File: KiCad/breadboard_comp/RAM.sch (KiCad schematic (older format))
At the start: 19 parts, among them SW9 SW_Push, U100 74LS00, U101 74LS245, U102 74LS245, U103 IDT6116SA, U104 IDT6116SA, U105 74LS00, U106 74LS245, U107 74LS245, U28 74LS08, U37 74LS32, U38 74LS08, U66 74LS00, U97 74LS08, U98 74LS32, U99 74LS08

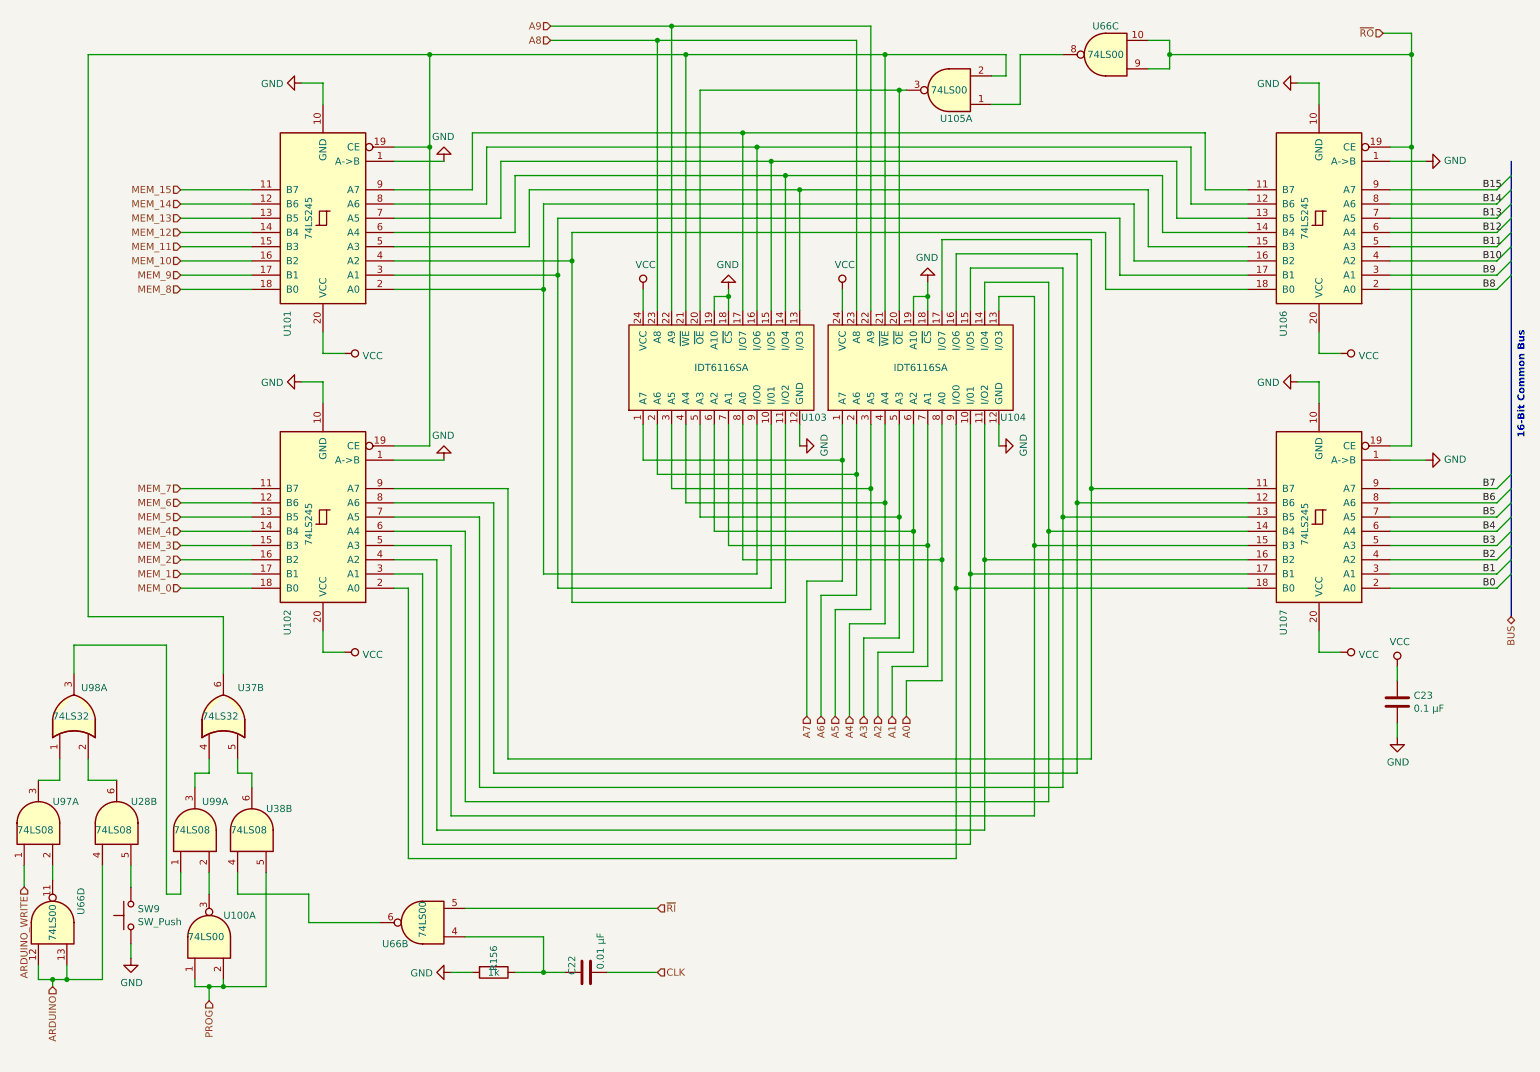
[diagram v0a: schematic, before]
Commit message: Computer built
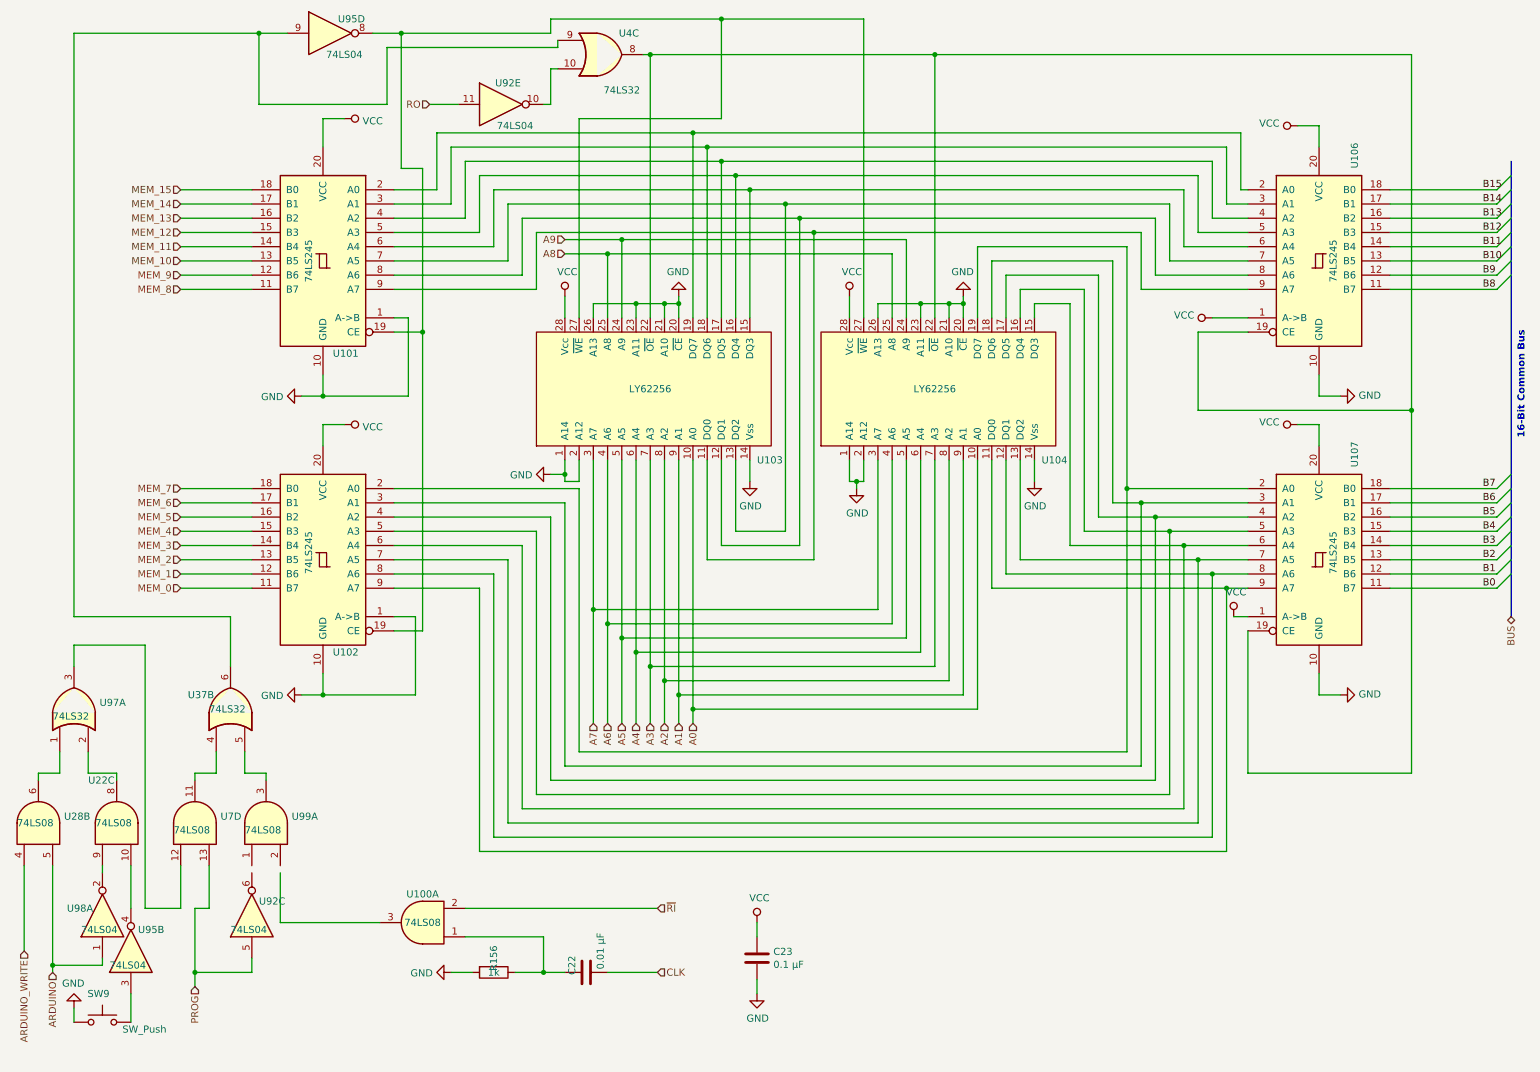
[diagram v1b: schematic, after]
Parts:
- removed U100, U105, U66: 74LS00, symbol 74xx:74LS00
- removed U103, U104: IDT6116SA, Package_DIP:DIP-24_W10.16mm_LongPads, symbol IDT_RAM:IDT6116SA
- removed U38, U97: 74LS08, symbol 74xx:74LS08
- removed U98: 74LS32, symbol 74xx:74LS32
- added U100, U22, U7: 74LS08, symbol 74xx:74LS08
- added U103, U104: LY62256, Package_DIP:DIP-28_W15.24mm, symbol IDT_RAM:LY62256
- added U4, U97: 74LS32, symbol 74xx:74LS32
- added U92, U95, U98: 74LS04, symbol 74xx:74LS04
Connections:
- net A0: now also U103.10 (A0), U104.10 (A0)
- net A1: now also U103.9 (A1), U104.9 (A1)
- net A2: now also U103.8 (A2), U104.8 (A2)
- net A3: now also U103.7 (A3), U104.7 (A3)
- net A4: now also U103.6 (A4), U104.6 (A4)
- net A5: now also U103.5 (A5), U104.5 (A5)
- net A6: now also U103.4 (A6), U104.4 (A6)
- net A7: now also U103.3 (A7), U104.3 (A7)
- net A8: now also U103.25 (A8), U104.25 (A8)
- net A9: now also U103.24 (A9), U104.24 (A9)
- net ARDUINO: now also U28.5, U98.1; no longer U28.4
- net ARDUINO_WRITE: now also U28.4
- net B0: now also U107.11 (B7); no longer U107.2 (A0)
- net B1: now also U107.12 (B6); no longer U107.3 (A1)
- net B10: now also U106.13 (B5); no longer U106.4 (A2)
- net B11: now also U106.14 (B4); no longer U106.5 (A3)
- net B12: now also U106.15 (B3); no longer U106.6 (A4)
- net B13: now also U106.16 (B2); no longer U106.7 (A5)
- net B14: now also U106.17 (B1); no longer U106.8 (A6)
- net B15: now also U106.18 (B0); no longer U106.9 (A7)
- net B2: now also U107.13 (B5); no longer U107.4 (A2)
- net B3: now also U107.14 (B4); no longer U107.5 (A3)
- net B4: now also U107.15 (B3); no longer U107.6 (A4)
- net B5: now also U107.16 (B2); no longer U107.7 (A5)
- net B6: now also U107.17 (B1); no longer U107.8 (A6)
- net B7: now also U107.18 (B0); no longer U107.9 (A7)
- net B8: now also U106.11 (B7); no longer U106.2 (A0)
- net B9: now also U106.12 (B6); no longer U106.3 (A1)
- net GND: now also U103.1 (A14), U103.14 (Vss), U103.2 (A12), U103.20 (~CE), U103.21 (A10), U103.23 (A11), U103.26 (A13), U104.1 (A14), U104.14 (Vss), U104.2 (A12), U104.20 (~CE), U104.21 (A10), U104.23 (A11), U104.26 (A13); no longer U106.1 (A->B), U107.1 (A->B)
- net MEM_0: now also U102.11 (B7); no longer U102.18 (B0)
- net MEM_1: now also U102.12 (B6); no longer U102.17 (B1)
- net MEM_10: now also U101.13 (B5); no longer U101.16 (B2)
- net MEM_11: now also U101.14 (B4); no longer U101.15 (B3)
- net MEM_12: now also U101.15 (B3); no longer U101.14 (B4)
- net MEM_13: now also U101.16 (B2); no longer U101.13 (B5)
- net MEM_14: now also U101.17 (B1); no longer U101.12 (B6)
- net MEM_15: now also U101.18 (B0); no longer U101.11 (B7)
- net MEM_2: now also U102.13 (B5); no longer U102.16 (B2)
- net MEM_3: now also U102.14 (B4); no longer U102.15 (B3)
- net MEM_4: now also U102.15 (B3); no longer U102.14 (B4)
- net MEM_5: now also U102.16 (B2); no longer U102.13 (B5)
- net MEM_6: now also U102.17 (B1); no longer U102.12 (B6)
- net MEM_7: now also U102.18 (B0); no longer U102.11 (B7)
- net MEM_8: now also U101.11 (B7); no longer U101.18 (B0)
- net MEM_9: now also U101.12 (B6); no longer U101.17 (B1)
- net PROG: now also U7.13, U92.5
- net VCC: now also U106.1 (A->B), U107.1 (A->B), U103.28 (Vcc), U104.28 (Vcc)
- net ~RI: now also U100.2
- net at U101.3 (A1): now also U106.3 (A1), U103.18 (DQ6); no longer U106.17 (B1)
- net at U101.4 (A2): now also U106.4 (A2), U103.17 (DQ5); no longer U106.18 (B0)
- net at U101.5 (A3): now also U106.5 (A3), U103.16 (DQ4); no longer U106.15 (B3)
- net at U101.6 (A4): now also U106.6 (A4), U103.15 (DQ3); no longer U106.14 (B4)
- net at U101.7 (A5): now also U106.7 (A5), U103.13 (DQ2); no longer U106.13 (B5)
- net at U101.8 (A6): now also U106.8 (A6), U103.12 (DQ1); no longer U106.12 (B6)
- net at U101.9 (A7): now also U106.9 (A7), U103.11 (DQ0); no longer U106.11 (B7)
- net at U101.19 (CE), U102.19 (CE): now also U103.27 (~WE), U104.27 (~WE), U95.8; no longer U37.6
- net at U101.2 (A0): now also U106.2 (A0), U103.19 (DQ7); no longer U106.16 (B2)
- net at U102.3 (A1): now also U107.3 (A1), U104.18 (DQ6); no longer U107.17 (B1)
- net at U102.4 (A2): now also U107.4 (A2), U104.17 (DQ5); no longer U107.16 (B2)
- net at U102.5 (A3): now also U107.5 (A3), U104.16 (DQ4); no longer U107.15 (B3)
- net at U102.6 (A4): now also U107.6 (A4), U104.15 (DQ3); no longer U107.14 (B4)
- net at U102.7 (A5): now also U107.7 (A5), U104.13 (DQ2); no longer U107.13 (B5)
- net at U102.8 (A6): now also U107.8 (A6), U104.12 (DQ1); no longer U107.12 (B6)
- net at U102.9 (A7): now also U107.9 (A7), U104.11 (DQ0); no longer U107.11 (B7)
- net at U102.2 (A0): now also U107.2 (A0), U104.19 (DQ7); no longer U107.18 (B0)
- net at C22.2, R156.1: now also U100.1
- net at SW9.2: now also U95.3; no longer U28.5
- net at U28.6: now also U97.1
- net at U37.4: now also U7.11; no longer U99.3
- net at U37.5: now also U99.3
- net ~RO: no longer names the net of U106.19 (CE), U107.19 (CE)
- net ~RO: now also U103.22 (~OE), U104.22 (~OE), U4.8
- new net: U22.10, U95.4
- new net: U22.8, U97.2
- new net: U22.9, U98.2
- new net: U7.12, U97.3
- new net: U37.6, U4.9, U95.9
- new net: U4.10, U92.10
- new net RO: U92.11
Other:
- moved on the sheet: C23, SW9, U101, U102, U106, U107

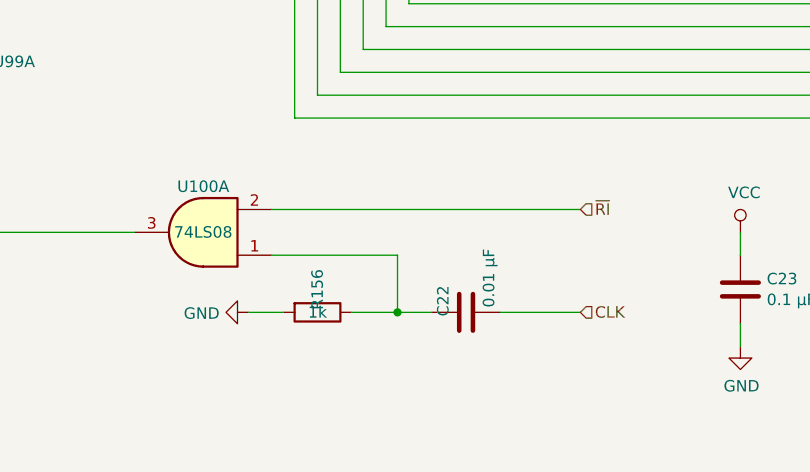
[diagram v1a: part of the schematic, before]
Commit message: Report Progress
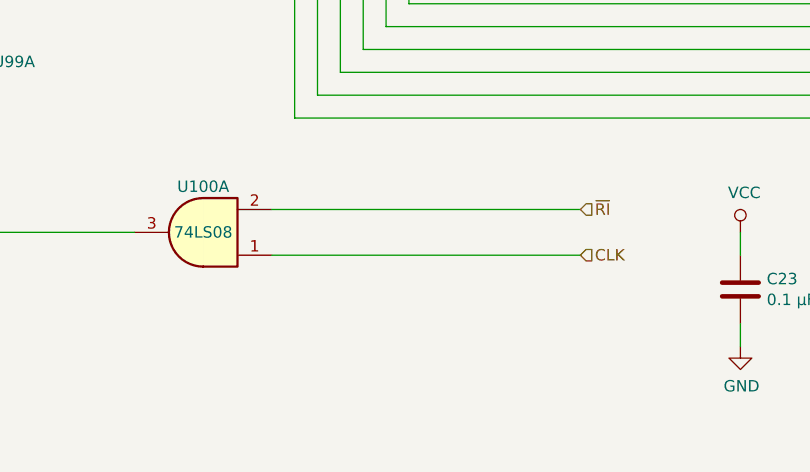
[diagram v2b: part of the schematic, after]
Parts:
- removed C22: 0.01 μF, symbol Device:C
- removed R156: 1k, symbol Device:R
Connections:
- net CLK: now also U100.1
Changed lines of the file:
@@
 Wire Wire Line
 	2200 4600 1700 4600
-Text HLabel 5050 7300 2    50   Input ~ 0
+Text HLabel 5050 7050 2    50   Input ~ 0
 CLK
 Text HLabel 5050 6850 2    50   Input ~ 0
 ~RI
-$Comp
-L Device:C C22
-U 1 1 602CA653
-P 4550 7300
-F 0 "C22" H 4500 7200 50  0000 C CNN
-F 1 "0.01 μF" H 4400 7400 50  0000 C CNN
-F 2 "" H 4588 7150 50  0001 C CNN
-F 3 "~" H 4550 7300 50  0001 C CNN
-	1    4550 7300
-	0    1    1    0
-$EndComp
-$Comp
-L Device:R R156
-U 1 1 602CB23C
-P 3900 7300
-F 0 "R156" H 3800 7300 50  0000 C CNN
-F 1 "1k" V 3900 7300 50  0000 C CNN
-F 2 "" V 3830 7300 50  0001 C CNN
-F 3 "~" H 3900 7300 50  0001 C CNN
-	1    3900 7300
-	0    1    1    0
-$EndComp
-Wire Wire Line
-	4050 7300 4250 7300
-Wire Wire Line
-	4700 7300 5050 7300
-$Comp
-L power:GND #PWR0258
-U 1 1 602FBBBF
-P 3600 7300
-F 0 "#PWR0258" H 3600 7050 50  0001 C CNN
-F 1 "GND" V 3605 7172 50  0000 R CNN
-F 2 "" H 3600 7300 50  0001 C CNN
-F 3 "" H 3600 7300 50  0001 C CNN
-	1    3600 7300
-	0    1    1    0
-$EndComp
-Wire Wire Line
-	3600 7300 3750 7300
-Wire Wire Line
-	3700 7050 4250 7050
-Wire Wire Line
-	4250 7050 4250 7300
-Connection ~ 4250 7300
-Wire Wire Line
-	4250 7300 4400 7300
 Text HLabel 1800 7400 3    50   Input ~ 0
 PROG
@@
 Wire Wire Line
 	5500 600  6500 600
+Wire Wire Line
+	3700 7050 5050 7050
 Wire Bus Line
 	11050 1600 11050 4800
